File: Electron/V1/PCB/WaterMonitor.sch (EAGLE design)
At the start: 36 parts, among them U1 SN74LV8154PW, U2 ELECTRONDUALNAMED, U3 24LC512, U4 DS1820SOIC

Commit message: Tidy up
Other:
- note added: "NB: Should these be pulled high as they are active low."
- moved on the sheet: C1, C2, C3, C4, C5, C6, CONN1, D1, D2, D3, H1, H2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

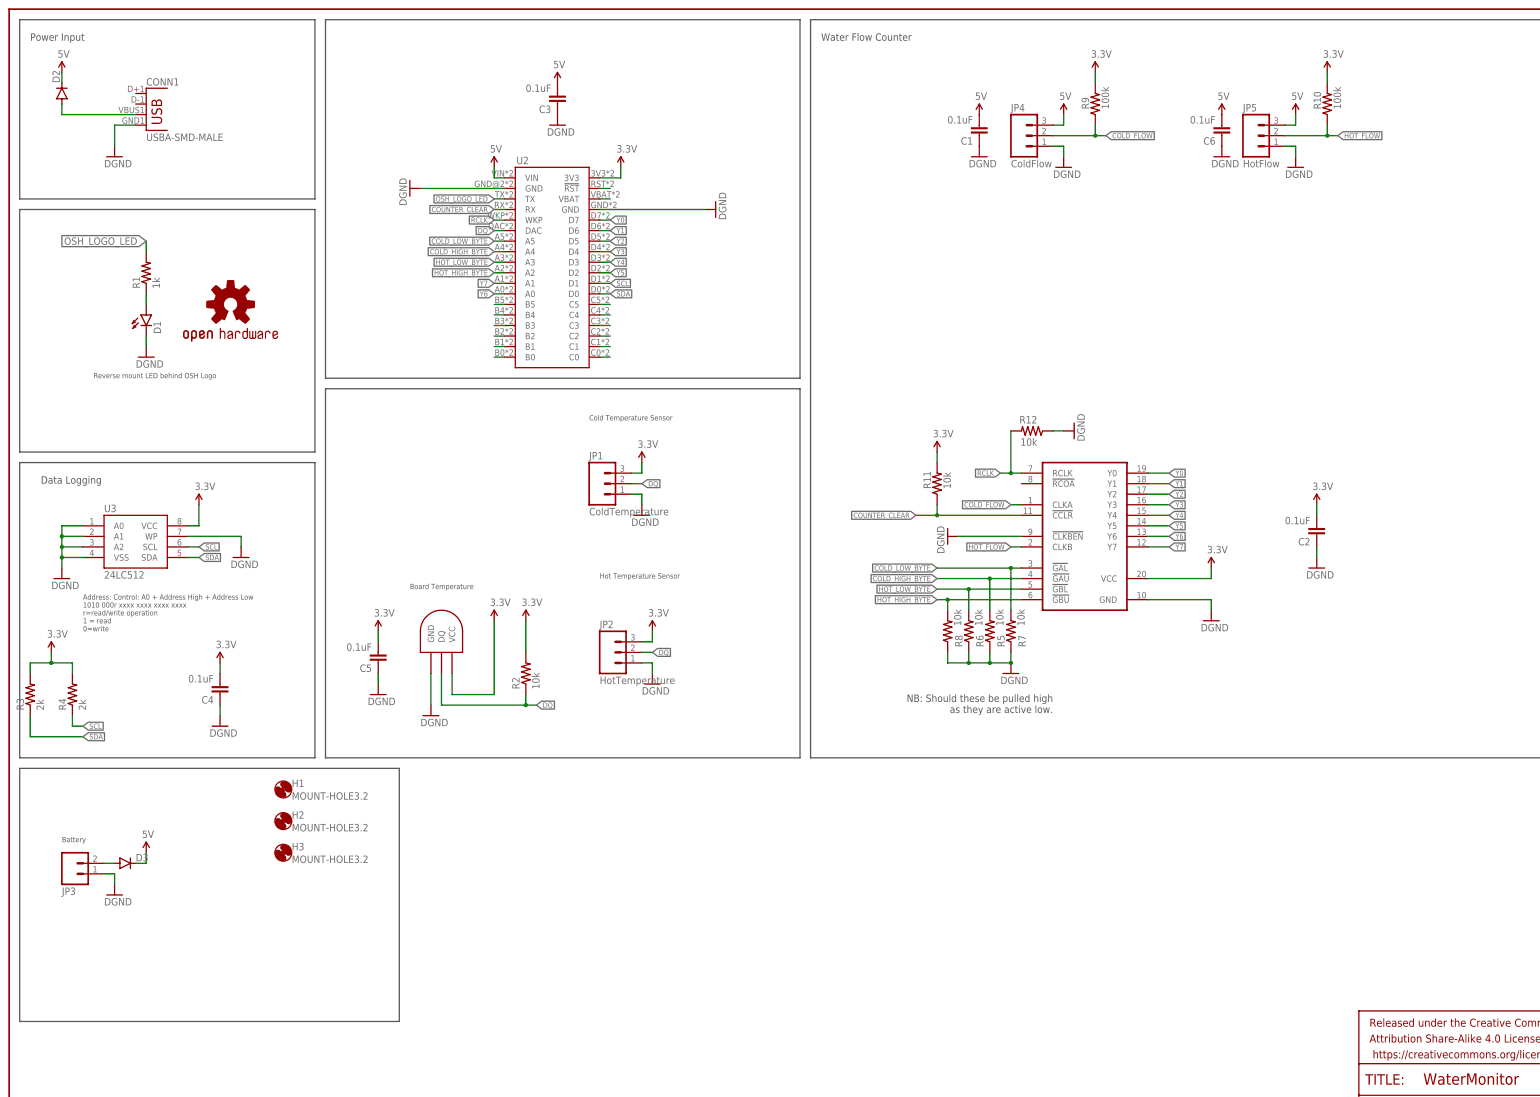
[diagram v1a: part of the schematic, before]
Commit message: V1.1 changes - not sure what. Not important - not using this version any more.
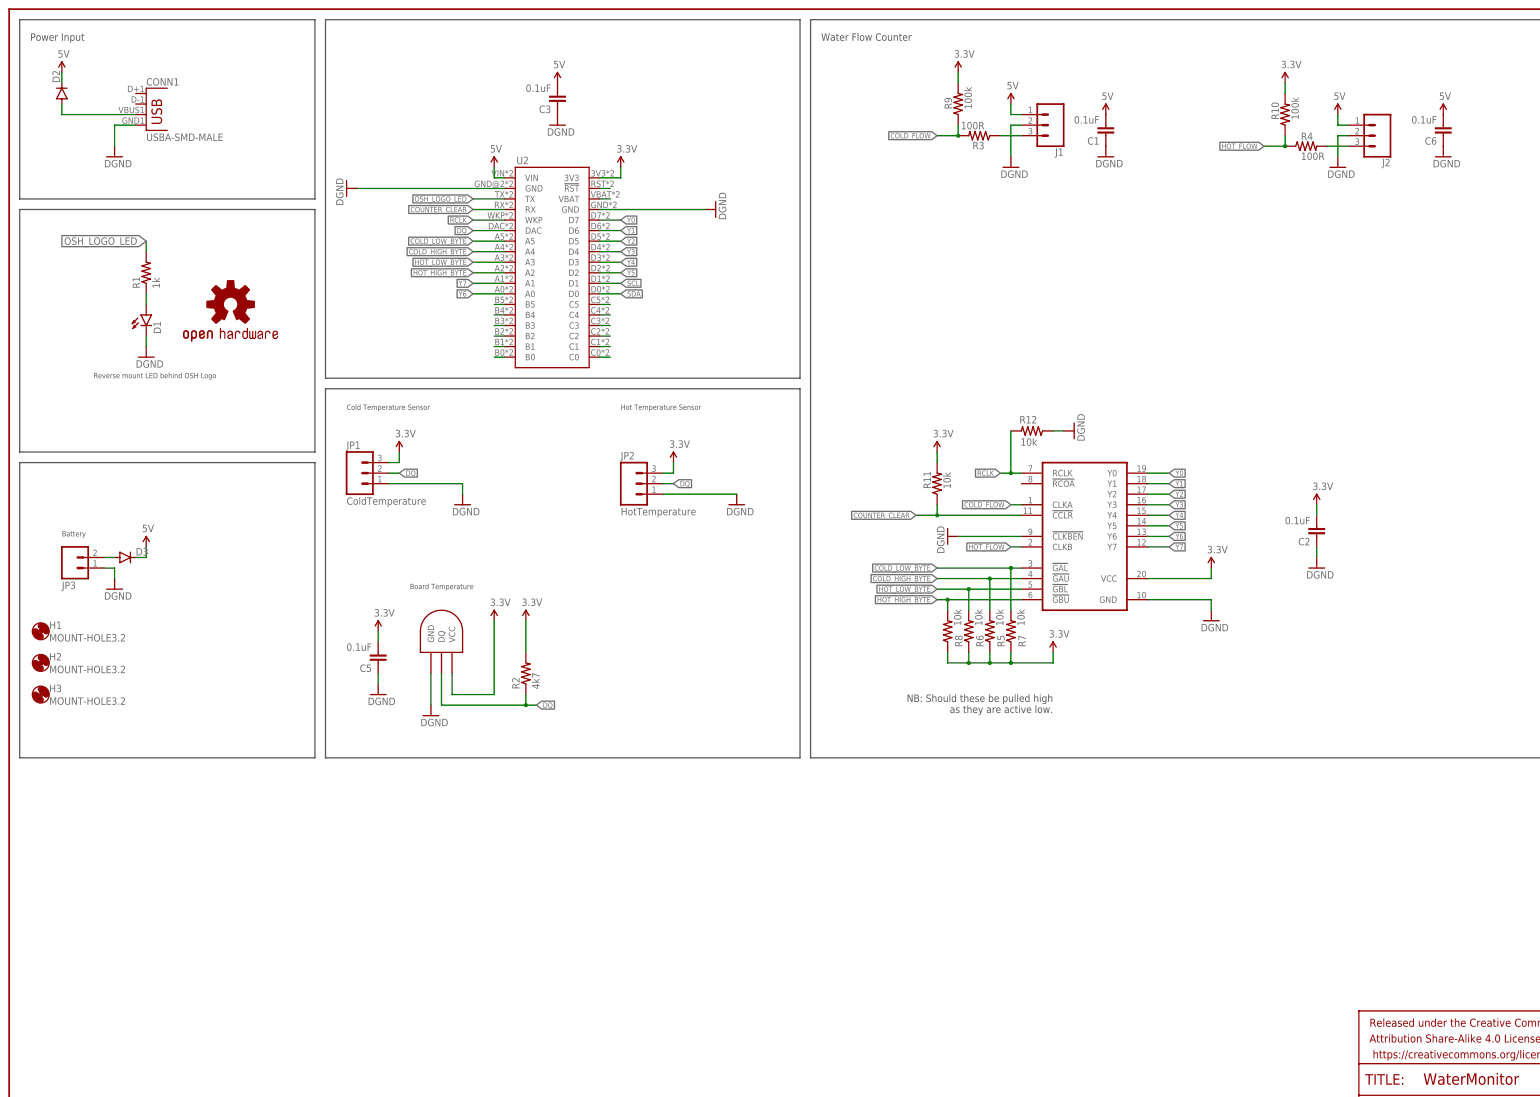
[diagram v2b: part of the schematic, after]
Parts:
- removed C4: 0.1uF, SparkFun-Passives:CAP0805
- removed JP4: ColdFlow, SparkFun-Connectors:M03POLAR
- removed JP5: HotFlow, SparkFun-Connectors:M03POLAR
- removed U3: 24LC512, SparkFun-DigitalIC:EEPROM-I2CSMD
- added J1, J2: (no value), Tinamous:CONN_03JST-HX-PTH-VERT
- R2: value 10k -> 4k7
- R3, R4: value 2k -> 100R
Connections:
- new net N$3: J1.3, R3.1
- new net N$4: J2.3, R4.2
- net 3.3V: now also R5.1, R6.1, R7.1, R8.1; no longer C4.2, R3.2, R4.2, U3.VCC
- net 5V: now also J1.1, J2.1; no longer JP4.3, JP5.3
- net COLD_FLOW: now also R3.2; no longer JP4.2
- net GND: now also J1.2, J2.2; no longer C4.1, JP4.1, JP5.1, R5.1, R6.1, R7.1, R8.1, U3.A0, U3.A1, U3.A2, U3.VSS, U3.WP
- net HOT_FLOW: now also R4.1; no longer JP5.2
- net SCL: no longer R4.1, U3.SCL
- net SDA: no longer R3.1, U3.SDA
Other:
- note removed: "1010 000r xxxx xxxx xxxx xxxx r=read/write operation 1 = read 0=write"
- note removed: "Address: Control: A0 + Address High + Address Low"
- note removed: "Data Logging"
- moved on the sheet: C1, C6, D3, H1, H2, H3, JP1, JP2, JP3, R10, R3, R4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
